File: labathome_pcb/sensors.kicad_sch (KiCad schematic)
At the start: 30 parts, among them J16 BME280, J17 CCS811, J21 QWIIC, U12 BME680, U13 BME280, U15 CCS811, U19 DS18B20, U20 BH1750, U22 AM612, U23 MPU-6050, U26 MSM261D4030H1CPM, U3 AHT21, U7 DS18B20, X2 XGZP6897D

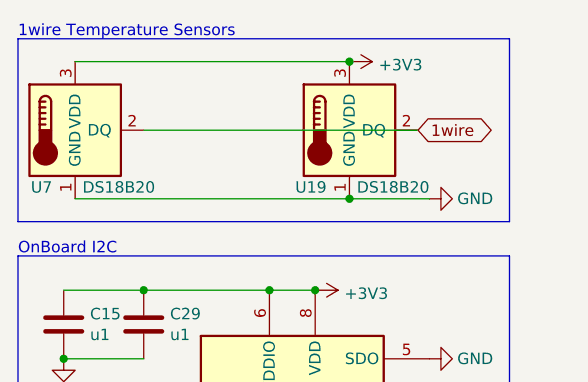
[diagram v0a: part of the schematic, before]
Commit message: Modbus Firmware
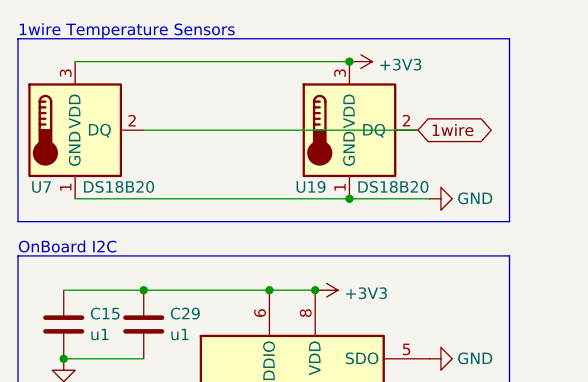
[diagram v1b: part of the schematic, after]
